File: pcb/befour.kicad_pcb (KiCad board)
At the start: 2 copper layers, 1 part

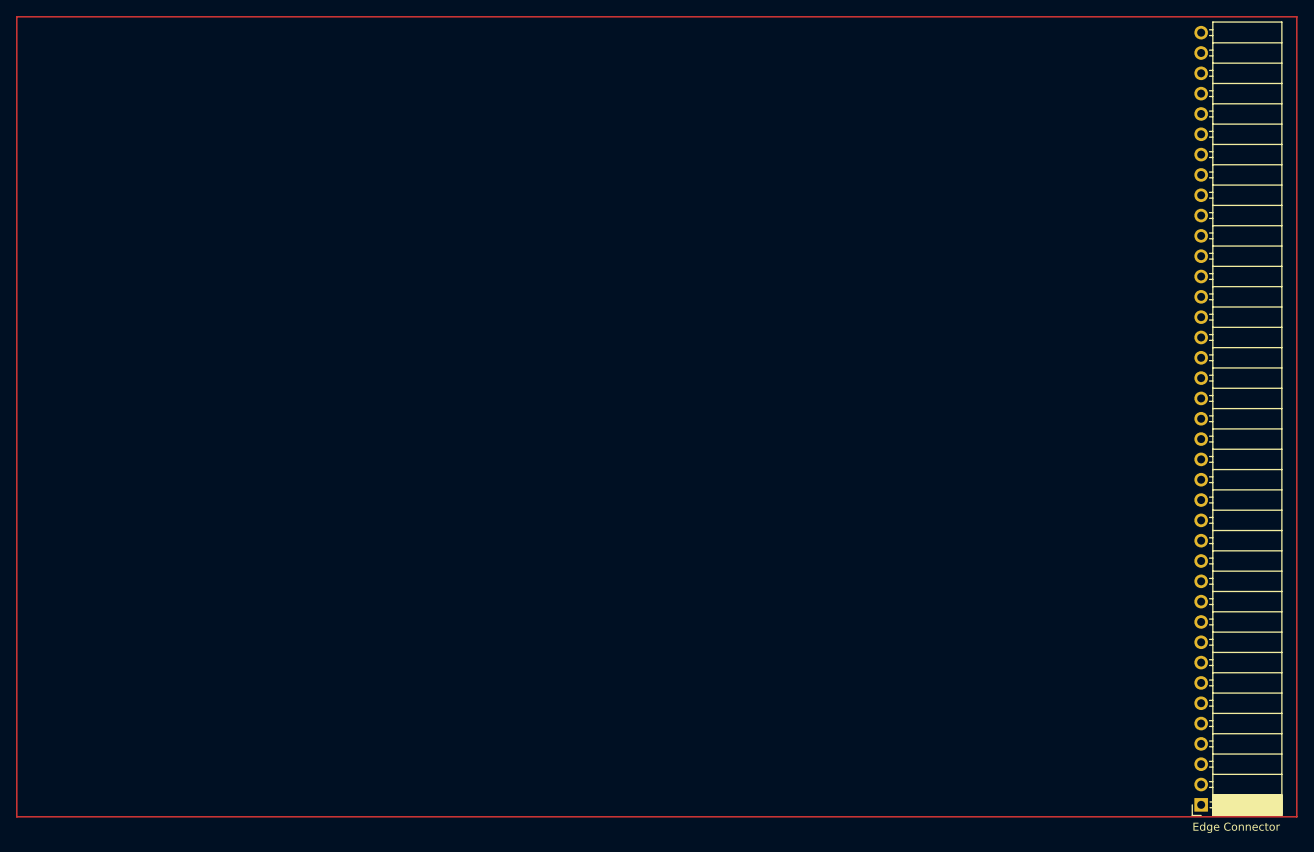
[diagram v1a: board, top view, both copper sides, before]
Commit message: more pcb work
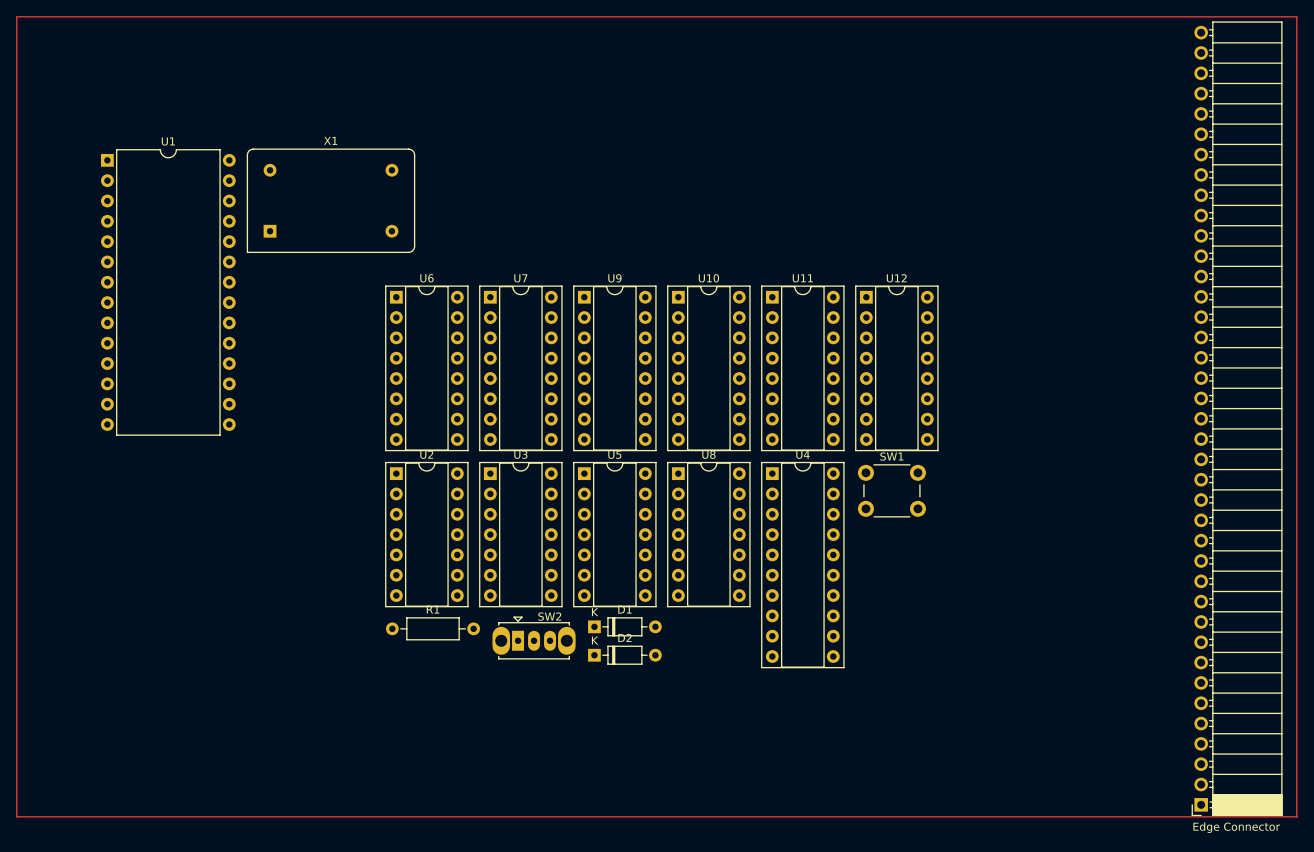
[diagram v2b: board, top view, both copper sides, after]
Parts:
- added D1: D, Diode_THT:D_DO-35_SOD27_P7.62mm_Horizontal, F.Cu at (123.6, 102.3)
- added D2: D, Diode_THT:D_DO-35_SOD27_P7.62mm_Horizontal, F.Cu at (123.6, 105.8)
- added R1: 10k, Resistor_THT:R_Axial_DIN0207_L6.3mm_D2.5mm_P10.16mm_Horizontal, F.Cu at (98.4, 102.5)
- added SW1: SW_Push, Button_Switch_THT:SW_PUSH_6mm_H5mm, F.Cu at (157.6, 83.0)
- added SW2: SW_SPDT, Button_Switch_THT:SW_Slide_SPDT_Straight_CK_OS102011MS2Q, F.Cu at (114.1, 104.0)
- added U1: MEMORY, Package_DIP:DIP-28_W15.24mm, F.Cu at (62.8, 44.0)
- added U10: AREG, Package_DIP:DIP-16_W7.62mm_Socket, F.Cu at (134.1, 61.1)
- added U11: TEMP, Package_DIP:DIP-16_W7.62mm_Socket, F.Cu at (145.9, 61.1)
- added U12: BREG, Package_DIP:DIP-16_W7.62mm_Socket, F.Cu at (157.6, 61.1)
- added U2: 74LS125, Package_DIP:DIP-14_W7.62mm_Socket, F.Cu at (98.9, 83.1)
- added U3: 74LS125, Package_DIP:DIP-14_W7.62mm_Socket, F.Cu at (110.6, 83.1)
- added U4: 74LS374, Package_DIP:DIP-20_W7.62mm_Socket, F.Cu at (145.9, 83.1)
- added U5: 74LS14, Package_DIP:DIP-14_W7.62mm_Socket, F.Cu at (122.4, 83.1)
- added U6: 74LS138, Package_DIP:DIP-16_W7.62mm_Socket, F.Cu at (98.9, 61.1)
- added U7: 74LS161, Package_DIP:DIP-16_W7.62mm_Socket, F.Cu at (110.6, 61.1)
- added U8: 74LS11, Package_DIP:DIP-14_W7.62mm_Socket, F.Cu at (134.1, 83.1)
- added U9: 74LS138, Package_DIP:DIP-16_W7.62mm_Socket, F.Cu at (122.4, 61.1)
- added X1: 1MHz, Oscillator:Oscillator_DIP-14, F.Cu at (83.1, 52.8)
